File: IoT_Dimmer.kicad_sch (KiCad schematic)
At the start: 42 parts, among them J1 Screw_Terminal_01x02, J2 Screw_Terminal_01x02, J3 Conn_01x06_Pin, U1 MOC3021M, U2 VOS628AT, U3 ESP32-C6FH4, Y2 Crystal_GND24

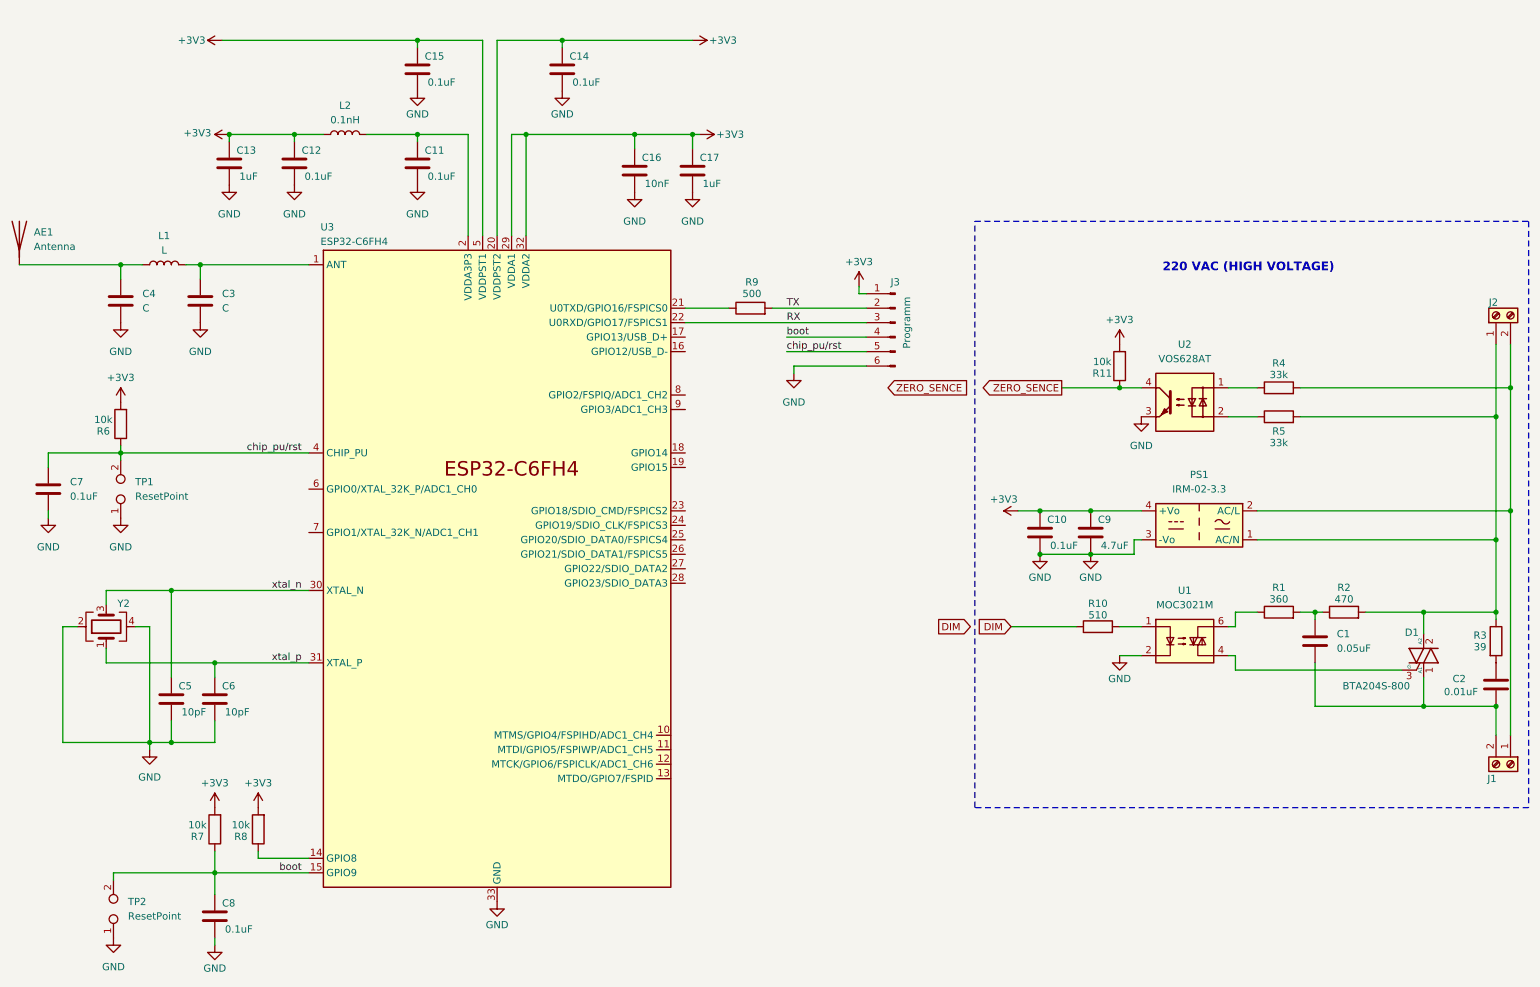
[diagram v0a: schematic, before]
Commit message: beta sheet
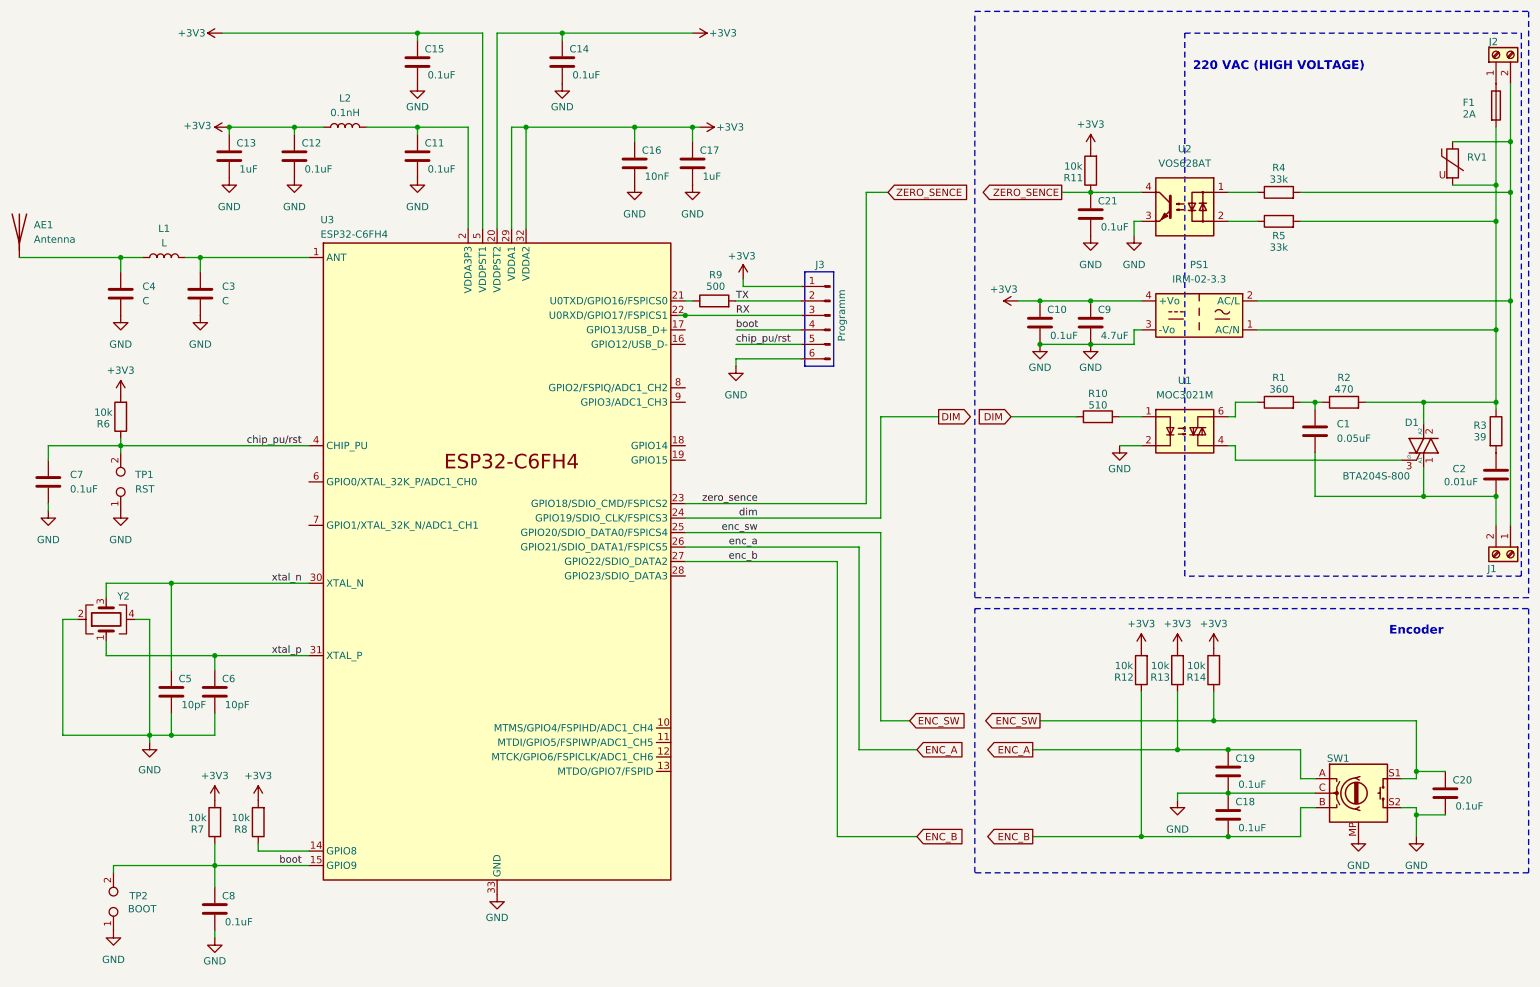
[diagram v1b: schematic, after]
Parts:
- added C18, C19, C20, C21: 0.1uF, symbol Device:C
- added F1: 2A, symbol Device:Fuse
- added R12, R13, R14: 10k, Resistor_SMD:R_0805_2012Metric, symbol Device:R
- added RV1: Varistor, Resistor_SMD:R_0805_2012Metric, symbol Device:Varistor
- added SW1: RotaryEncoder_Switch_MP, symbol Device:RotaryEncoder_Switch_MP
- AE1: footprint (none) -> RF_Antenna:Molex_47948-0001_2.4Ghz
- R1, R10, R11, R2, R3, R6, R7, R8, R9: footprint (none) -> Resistor_SMD:R_0805_2012Metric
- TP1: value ResetPoint -> RST; footprint (none) -> TestPoint:TestPoint_Bridge_Pitch2.0mm_Drill0.7mm
- TP2: value ResetPoint -> BOOT; footprint (none) -> TestPoint:TestPoint_Bridge_Pitch2.0mm_Drill0.7mm
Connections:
- net +3V3: now also R12.2, R13.2, R14.2
- net DIM: now also U3.24 (GPIO19/SDIO_CLK/FSPICS3)
- net GND: now also C18.1, C19.2, C20.2, C21.2, SW1.C, SW1.MP, SW1.S2
- net ZERO_SENCE: now also U3.23 (GPIO18/SDIO_CMD/FSPICS2), C21.1
- net at D1.2 (A2), PS1.1 (AC/N), R2.2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: now also F1.2, RV1.2; no longer J2.1 (Pin_1)
- net at J1.1 (Pin_1), J2.2 (Pin_2), PS1.2 (AC/L)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: now also RV1.1
- net ENC_SW: now reaches U3.25 (GPIO20/SDIO_DATA0/FSPICS4)
- net ENC_SW: now also C20.1, R14.1, SW1.S1
- net ENC_A: now reaches U3.26 (GPIO21/SDIO_DATA1/FSPICS5)
- net ENC_A: now also C19.1, R13.1, SW1.A
- net ENC_B: now reaches U3.27 (GPIO22/SDIO_DATA2)
- net ENC_B: now also C18.2, R12.1, SW1.B
- new net: F1.1, J2.1 (Pin_1)
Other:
- note added: "Encoder"
- moved on the sheet: AE1, C1, C10, C11, C12, C13, C14, C15, C16, C17, C2, C3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
